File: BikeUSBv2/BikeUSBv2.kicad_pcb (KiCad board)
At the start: 2 copper layers, 43.6 x 25.5 mm, 52 parts, among them J1 TYPE-C-31-M-16, J2 JST S2B-EH(LF)(SN), Q1 MMBT3906, SW1 1TS002E-2500-2501-CT, SW2 1TS002E-2500-2501-CT, U1 TPS63020DSJR, U2 ATtiny1616-M

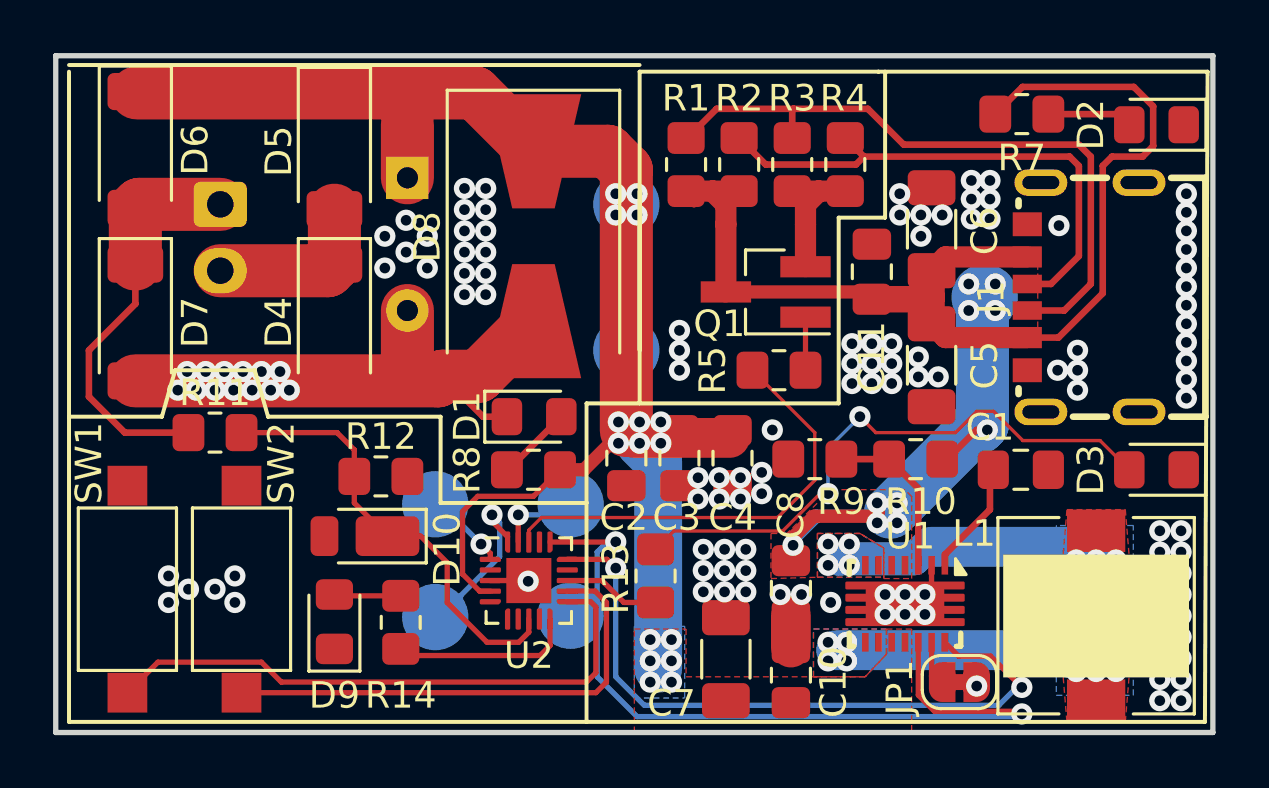
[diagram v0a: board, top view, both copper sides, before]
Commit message: stuff
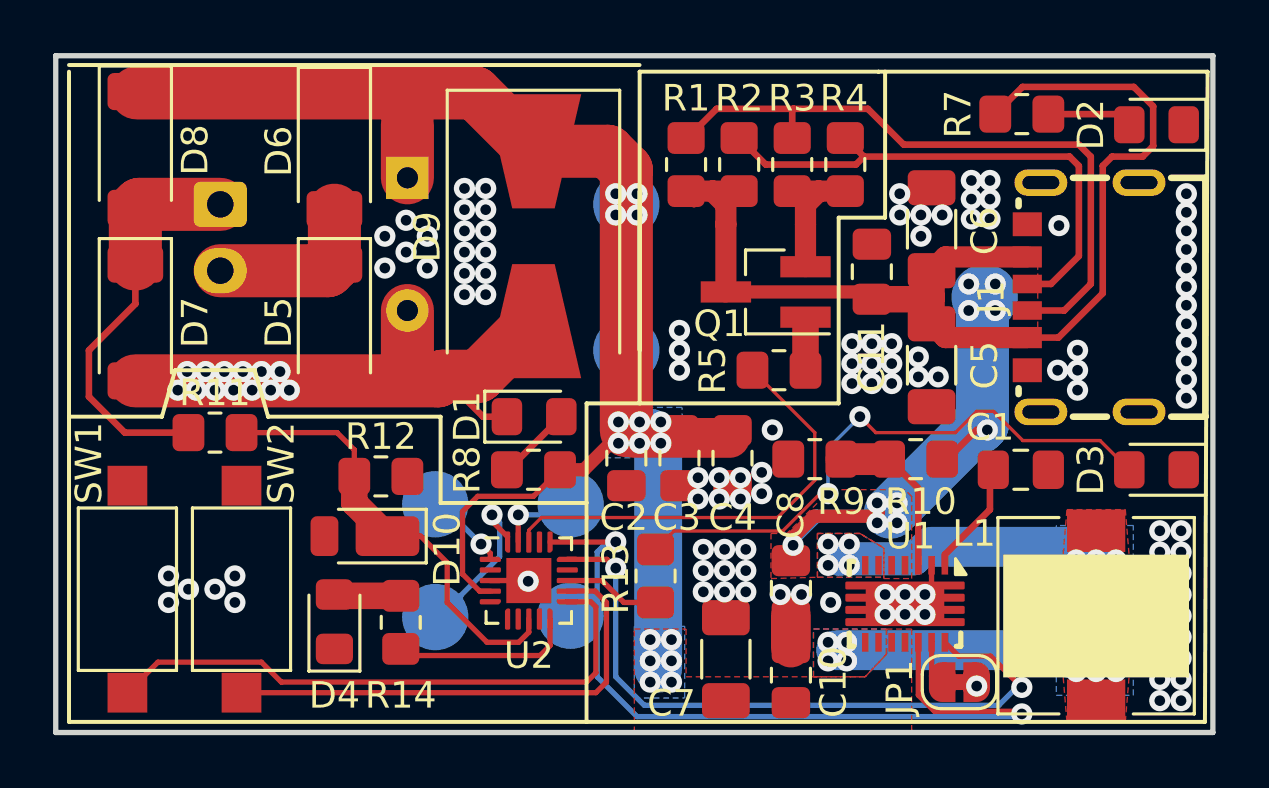
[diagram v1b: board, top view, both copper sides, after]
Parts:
- renumbered D9 to D4, D4 to D5, D5 to D6, D6 to D8, D8 to D9

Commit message: half capacitance, but cheaper
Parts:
- C9: value 1F -> 4700µF
